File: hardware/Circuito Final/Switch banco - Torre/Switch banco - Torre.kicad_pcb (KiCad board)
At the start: 2 copper layers, 98.6 x 48.6 mm, 69 parts, among them J1 Conn_01x07, J2 Conn_02x07_Odd_Even, J3 Conn_01x07, Q1 MMBFJ112, Q1_1 MMBT2222A, Q3 MMBT2222A, U1 74HC595, U2 74HC4051

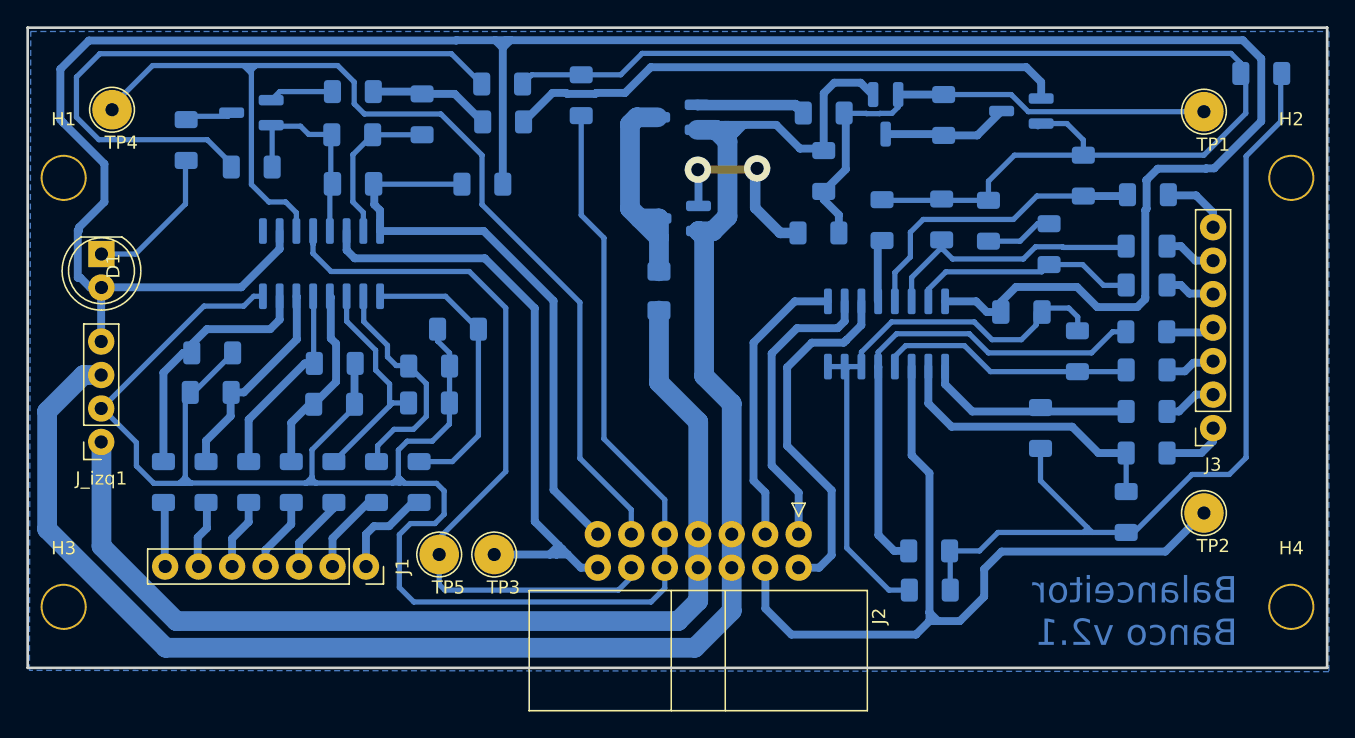
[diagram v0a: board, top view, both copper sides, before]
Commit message: version 2.2 Banco
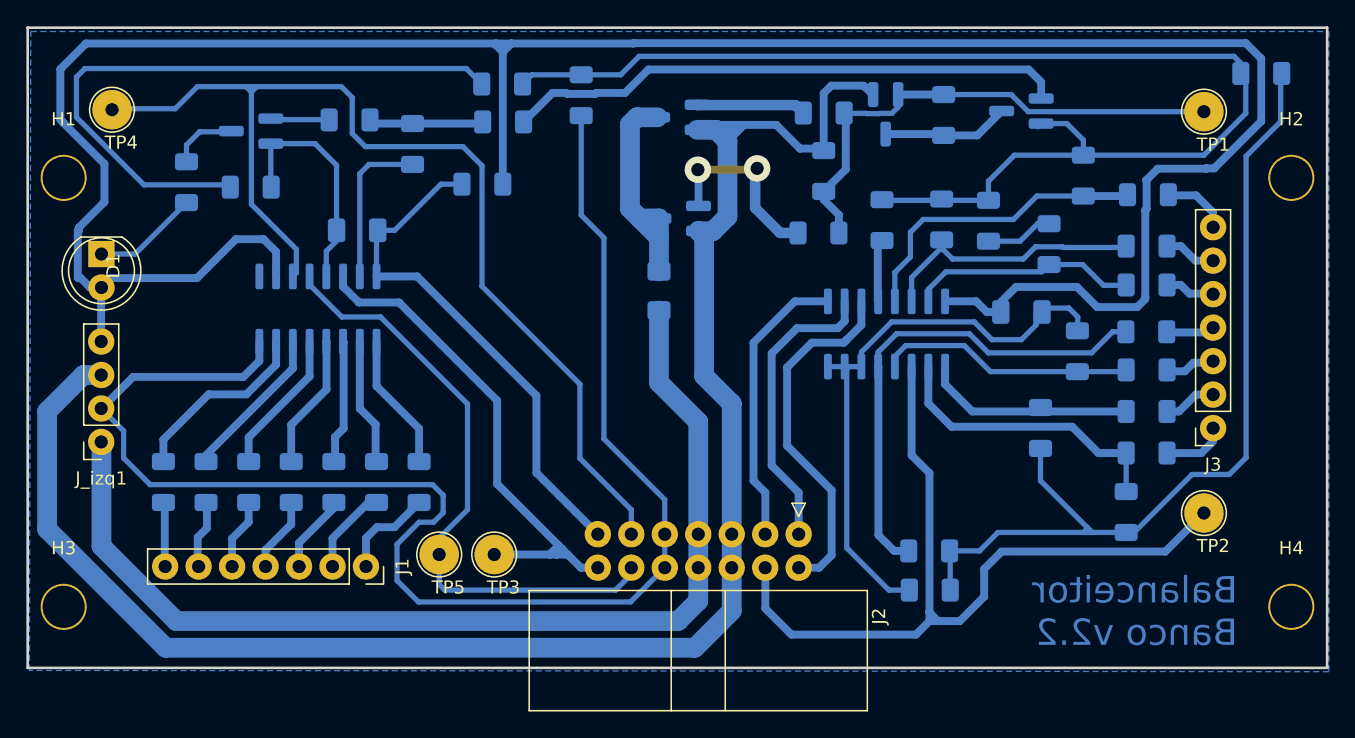
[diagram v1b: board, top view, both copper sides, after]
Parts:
- removed Rp1, Rp2, Rp3, Rp4, Rp5, Rp6, Rp7, Rp8: 10k, Resistor_SMD:R_1206_3216Metric_Pad1.30x1.75mm_HandSolder
- moved C1 3.54 mm to (125.1, 91.0)
- moved U1 3.46 mm to (122.1, 97.0)
- moved R5 3.20 mm to (112.2, 87.4)
- moved Rs8 2.36 mm to (129.3, 84.5)
- moved R4 2.16 mm to (124.5, 82.7)
- moved R2_13 1.53 mm to (117.0, 87.8)
- moved Q3 1.40 mm to (117.1, 83.5)
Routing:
- net GND: track 428.3 -> 387.8 mm
- net Net-(U1-QB): track 21.9 -> 10.4 mm
- net /latch: track 55.0 -> 44.0 mm
- net Net-(U1-QD): track 17.2 -> 9.30 mm
- net Net-(U1-QC): track 17.1 -> 9.53 mm
- net /DATA: track 47.1 -> 39.8 mm
- net /Vcc: track 232.8 -> 227.5 mm
- net Net-(U1-QH): track 19.4 -> 14.3 mm
- net Net-(U1-QG): track 15.9 -> 11.8 mm
- net Net-(U1-QF): track 14.9 -> 11.0 mm
- net Net-(U1-QE): track 14.0 -> 10.2 mm
- net Net-(D1-K): track 11.2 -> 8.07 mm
- net Net-(Q3-C): track 3.09 -> 5.04 mm
- net /Vbanco: track 9.01 -> 8.15 mm
- net /clock: track 82.7 -> 82.1 mm
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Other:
- board text added: "Balanceitor Banco v2.2"
- board text removed: "Balanceitor Banco v2.1"
